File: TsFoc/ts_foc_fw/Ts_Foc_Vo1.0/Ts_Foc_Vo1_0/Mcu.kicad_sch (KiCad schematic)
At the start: 8 parts, among them SW1 BOTTOM

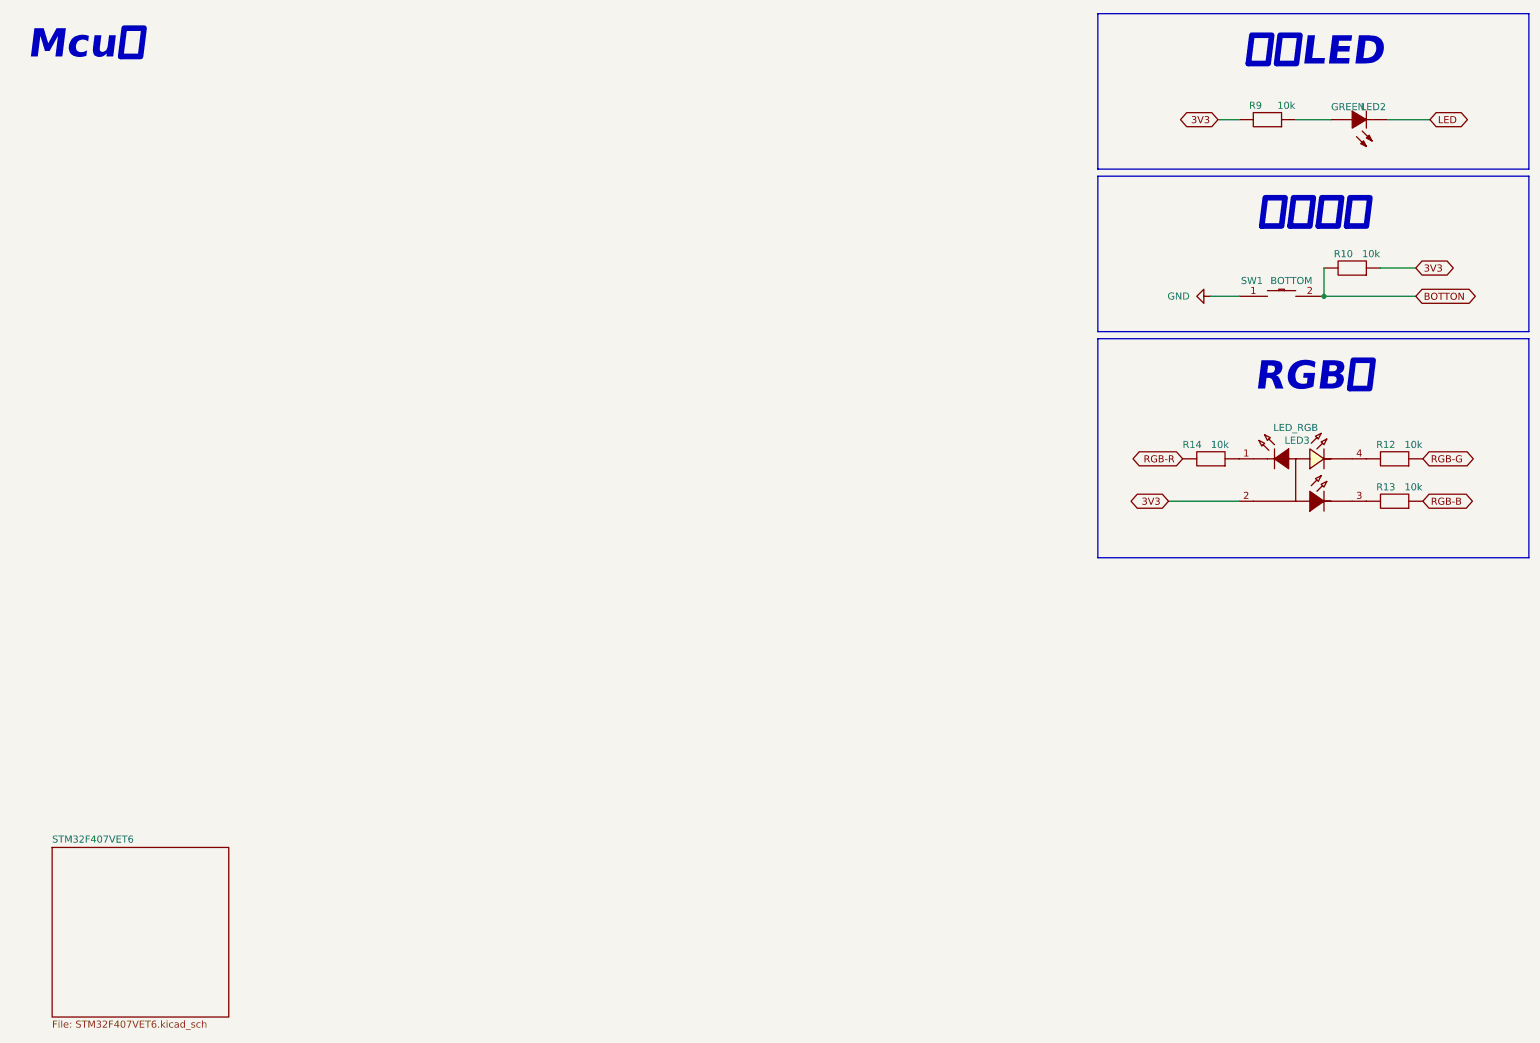
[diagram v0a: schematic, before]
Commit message: 同步_原理图小幅优化
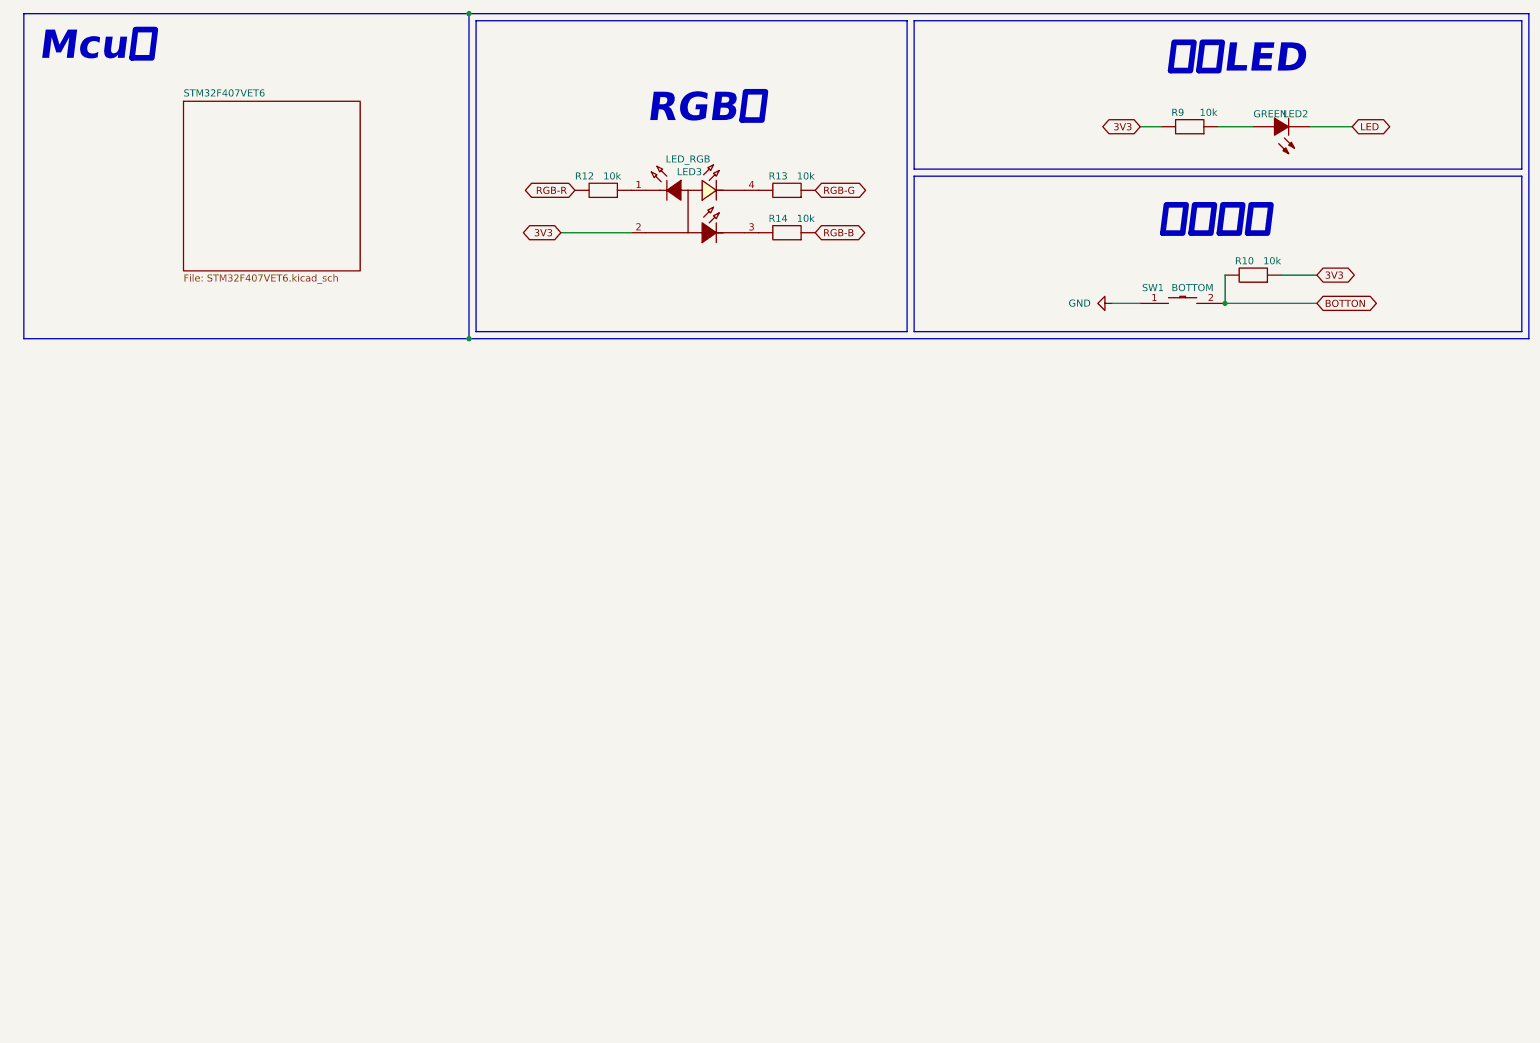
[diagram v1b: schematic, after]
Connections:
- net RGB-B: now also R14.1; no longer R13.1
- net RGB-G: now also R13.1; no longer R12.1
- net RGB-R: now also R12.2; no longer R14.2
- net at LED3.1 (R-): now also R12.1; no longer R14.1
- net at LED3.4 (G-): now also R13.2; no longer R12.2
- net at LED3.3 (B-): now also R14.2; no longer R13.2
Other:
- moved on the sheet: LED2, R10, R9, SW1
